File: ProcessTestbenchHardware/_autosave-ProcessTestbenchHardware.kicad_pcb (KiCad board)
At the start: 2 copper layers, 110 x 75 mm, 55 parts, among them J1 Fluxo1, J11 LSLL1, J12 LSHH2, J13 LSLL2, J14 Servo, J2 Fluxo2, J3 Fluxo3, J4 Pressao1, J5 Pressao2, J6 Term1, J7 Term2, J8 LSHH1, Q1 IRLZ44N, Q2 IRLZ44N, Q3 IRLZ44N, Q4 IRLZ44N, Q5 IRLZ44N, U2 MAX485E

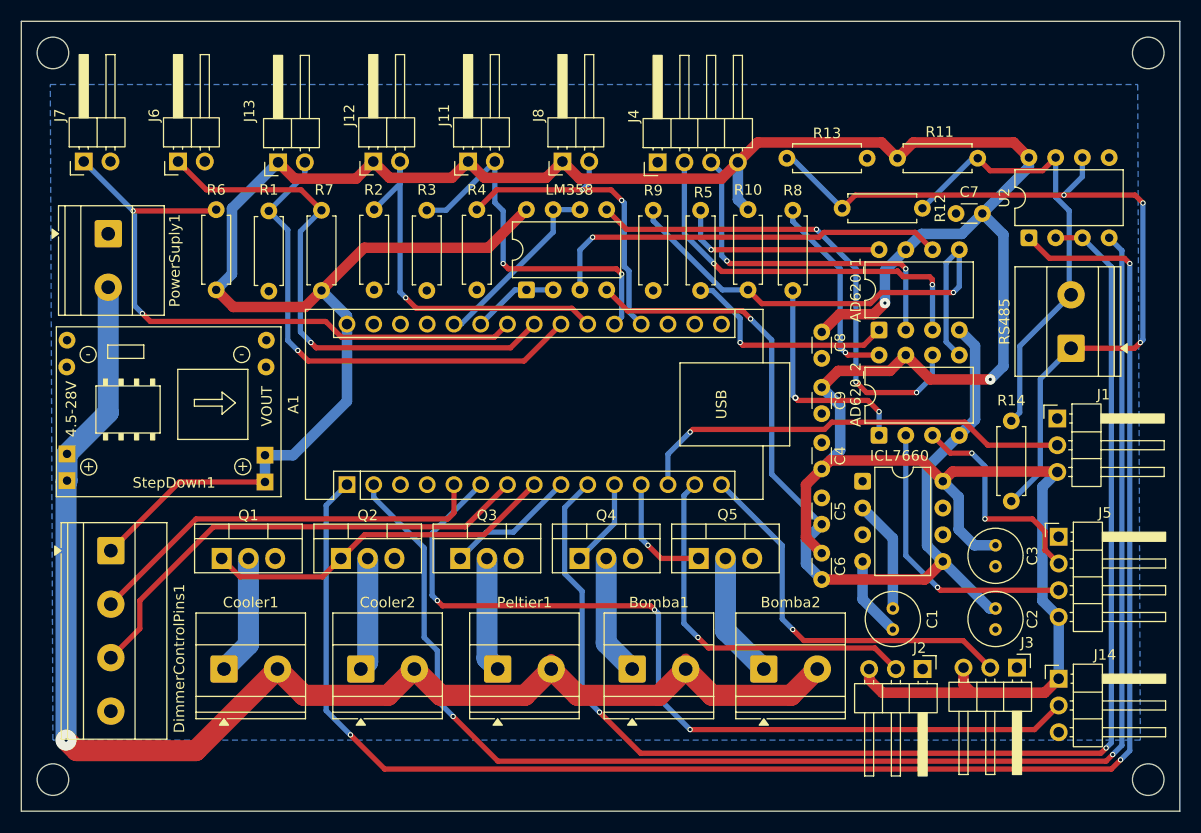
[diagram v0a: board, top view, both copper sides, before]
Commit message: Buttons, Servo and Thermistors Testing
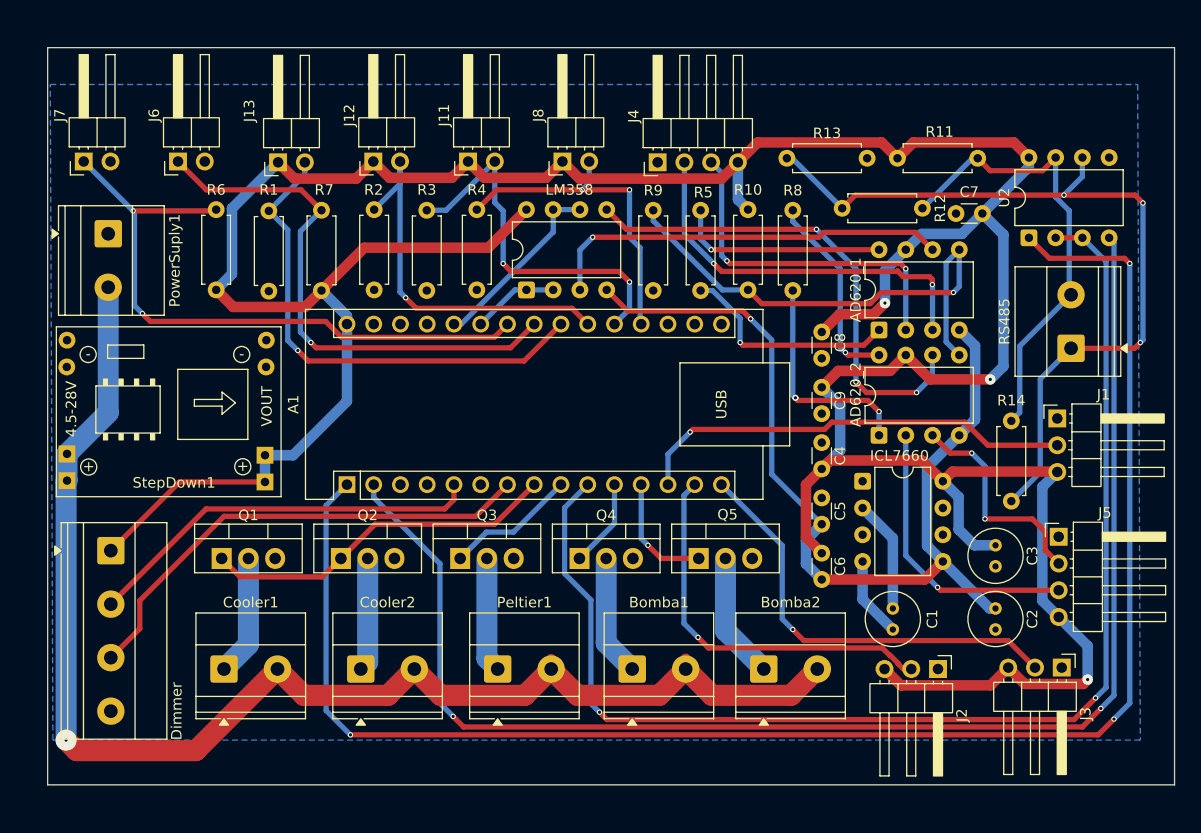
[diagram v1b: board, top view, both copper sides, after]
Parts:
- removed J14: Servo, Connector_PinHeader_2.54mm:PinHeader_1x03_P2.54mm_Horizontal
- J3: value Fluxo3 -> Fluxo
- moved J3 4.25 mm to (153.8, 105.4)
- moved J2 1.46 mm to (142.0, 105.5)
- renumbered DimmerControlPins1 to Dimmer
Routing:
- net /SaidaServoMotor: track 82.8 -> 0.00 mm, vias 3 -> 0
- net /MAX485_TX: track 139.7 -> 133.2 mm
- net /DE/RE_MAX485: track 126.1 -> 119.7 mm
- net /MAX485_RX: track 158.4 -> 153.1 mm
- net /Fluxo3: track 36.8 -> 41.1 mm
- net /Fluxo2: track 35.5 -> 37.0 mm
- net /LSHH1: track 30.5 -> 31.5 mm
- net /ZcDimmer: track 38.9 -> 38.1 mm
- net /LSLL1: track 35.1 -> 35.7 mm
- net +5V: track 333.3 -> 333.2 mm, vias 2 -> 3
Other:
- board size 110 x 75 mm -> 107 x 70 mm
